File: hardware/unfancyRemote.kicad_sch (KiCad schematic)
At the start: 50 parts, among them J3 HALL1/PPM, J4 HALL2, J6 VIN, J7 VBAT, J8 Motor, Q1 AO3401A, Q2 MMBT3904, Q3 MMBT3904, SW1 SW_Push, U1 E28-2G4M12S, U2 MCP73871-2AA, U3 ESP32-C3_SUPERMINI

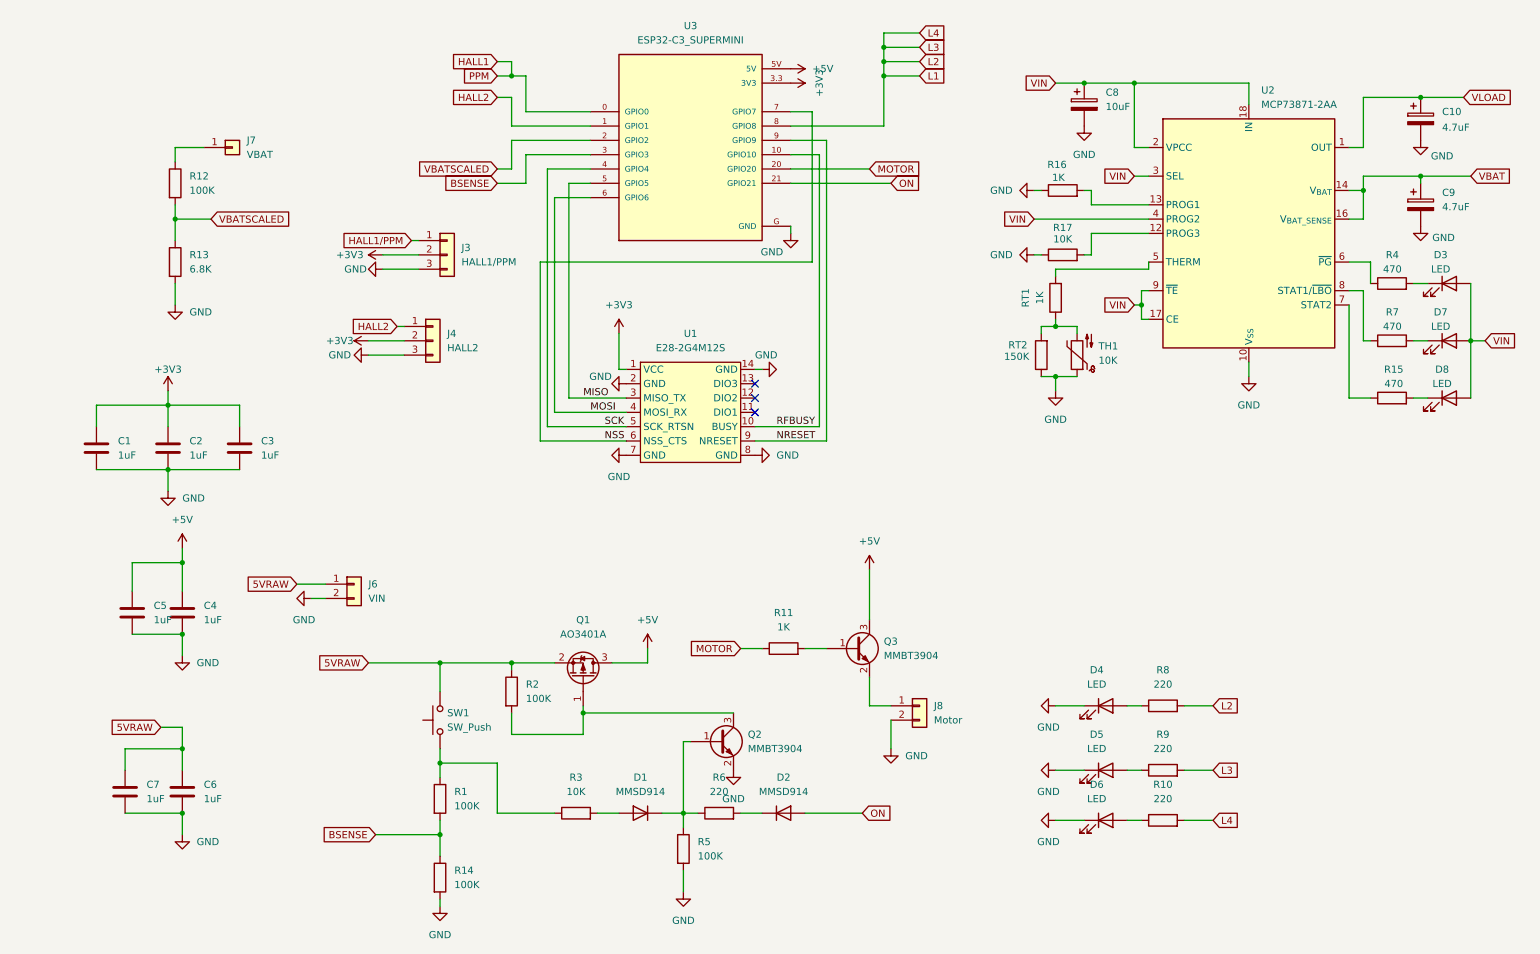
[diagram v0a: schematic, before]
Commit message: power progress
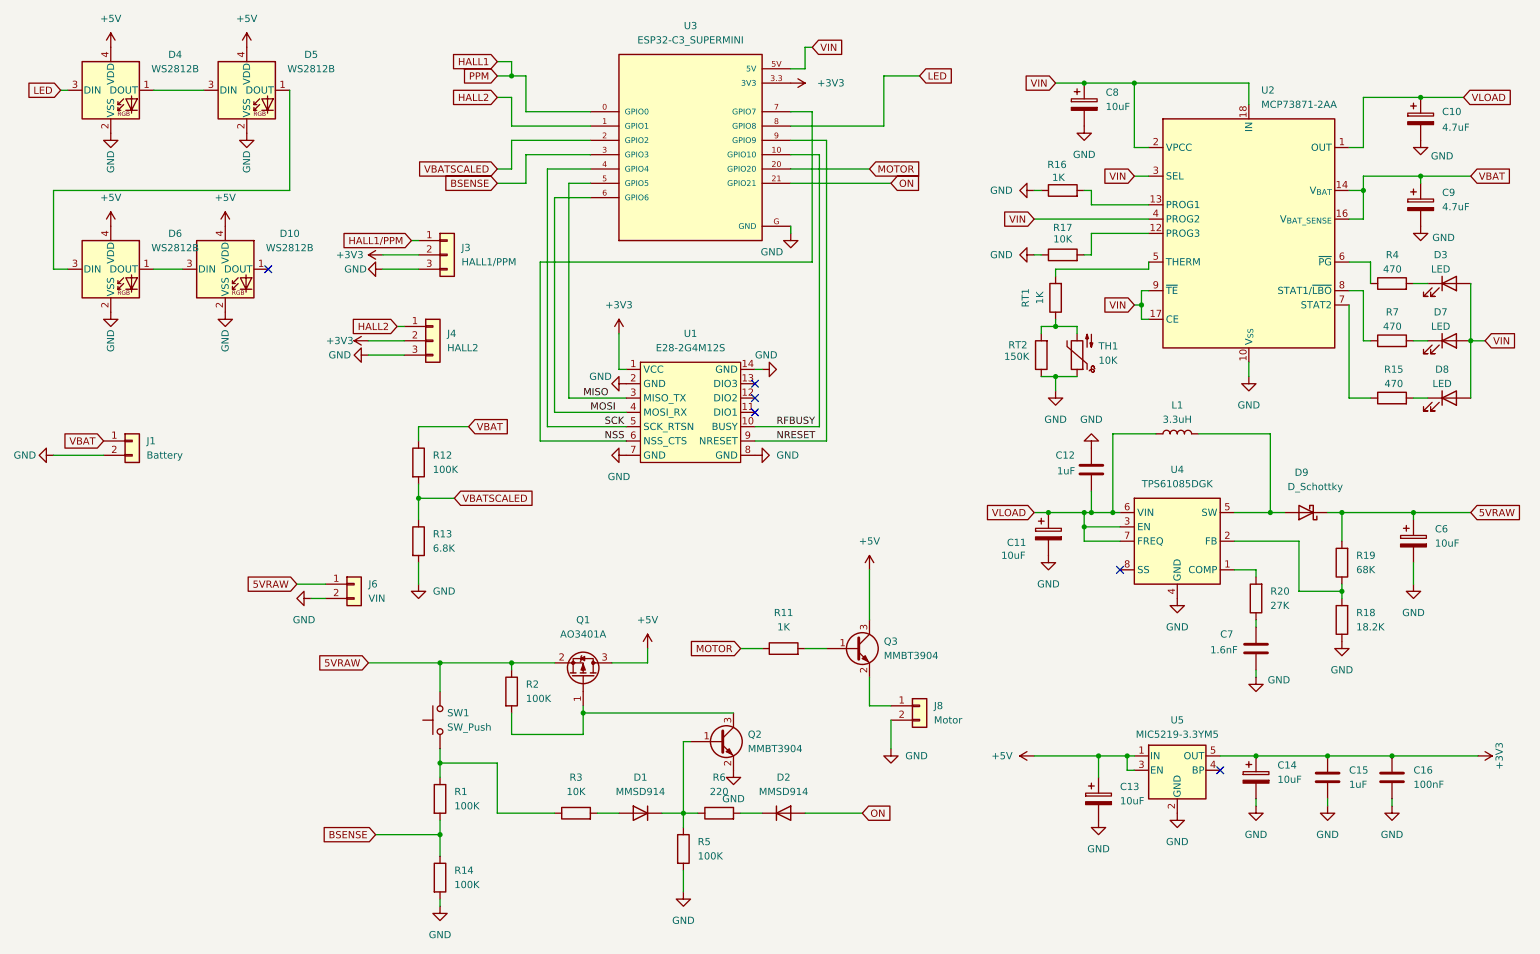
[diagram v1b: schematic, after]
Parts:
- removed C1, C2, C3, C4, C5, C6: 1uF, Capacitor_SMD:C_0603_1608Metric, symbol Device:C
- removed D4, D5, D6: LED, LED_SMD:LED_0805_2012Metric, symbol Device:LED
- removed J7: VBAT, Connector_wire:SolderWirePad_1x01_SMD_1x2mm, symbol Connector_Generic:Conn_01x01
- removed R10, R8, R9: 220, Resistor_SMD:R_0603_1608Metric, symbol Device:R
- added C11, C13, C14, C6: 10uF, Capacitor_Tantalum_SMD:CP_EIA-3216-10_Kemet-I, symbol Device:C_Polarized
- added C12, C15: 1uF, Capacitor_SMD:C_0402_1005Metric, symbol Device:C
- added C16: 100nF, Capacitor_SMD:C_0402_1005Metric, symbol Device:C
- added D10, D4, D5, D6: WS2812B, LED_SMD:LED_WS2812B-2020_PLCC4_2.0x2.0mm, symbol LED:WS2812B-2020
- added D9: D_Schottky, Diode_SMD:D_SOD-523, symbol Device:D_Schottky
- added J1: Battery, unfancyRemote_components:SolderWirePad_1x02_SMD_1x2mm, symbol Connector_Generic:Conn_01x02
- added L1: 3.3uH, Inductor_SMD:L_01005_0402Metric, symbol Device:L
- added R18: 18.2K, Resistor_SMD:R_0402_1005Metric, symbol Device:R
- added R19: 68K, Resistor_SMD:R_0402_1005Metric, symbol Device:R
- added R20: 27K, Resistor_SMD:R_0402_1005Metric, symbol Device:R
- added U4: TPS61085DGK, Package_SO:VSSOP-8_3x3mm_P0.65mm, symbol Regulator_Switching:TPS61085DGK
- added U5: MIC5219-3.3YM5, Package_TO_SOT_SMD:SOT-23-5, symbol Regulator_Linear:MIC5219-3.3YM5
- C10, C8, C9: footprint (none) -> Capacitor_Tantalum_SMD:CP_EIA-3216-10_Kemet-I
- C7: value 1uF -> 1.6nF; footprint Capacitor_SMD:C_0603_1608Metric -> Capacitor_SMD:C_0402_1005Metric
- R1, R11, R12, R13, R14, R15, R16, R17, R2, R3, R4, R5, R6, R7, RT1, RT2: footprint Resistor_SMD:R_0603_1608Metric -> Resistor_SMD:R_0402_1005Metric
- TH1: footprint (none) -> Resistor_SMD:R_0402_1005Metric
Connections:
- net +3V3: now also C14.1, C15.1, C16.1, U5.5 (OUT)
- net +5V: now also C13.1, D10.4 (VDD), D4.4 (VDD), D5.4 (VDD), D6.4 (VDD), U5.1 (IN), U5.3 (EN); no longer U3.5V
- net 5VRAW: now also C6.1, D9.1 (K), R19.2; no longer C7.1
- net GND: now also C11.2, C12.1, C13.2, C14.2, C15.2, C16.2, C6.2, D10.2 (VSS), D4.2 (VSS), D5.2 (VSS), D6.2 (VSS), J1.2 (Pin_2), R18.1, U4.4 (GND), U5.2 (GND)
- net VBAT: now also R12.1, J1.1 (Pin_1)
- net VIN: now also U3.5V
- net VLOAD: now also C11.1, C12.2, L1.1, U4.3 (EN), U4.6 (VIN), U4.7 (FREQ)
- net L1 renamed LED
- net LED: now also D4.3 (DIN)
- new net: R18.2, R19.1, U4.2 (FB)
- new net: C7.1, R20.1
- new net: D9.2 (A), L1.2, U4.5 (SW)
- new net: D10.3 (DIN), D6.1 (DOUT)
- new net: D4.1 (DOUT), D5.3 (DIN)
- new net: D5.1 (DOUT), D6.3 (DIN)
- new net: R20.2, U4.1 (COMP)
- no-connect marks 3 -> 6
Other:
- moved on the sheet: R12, R13

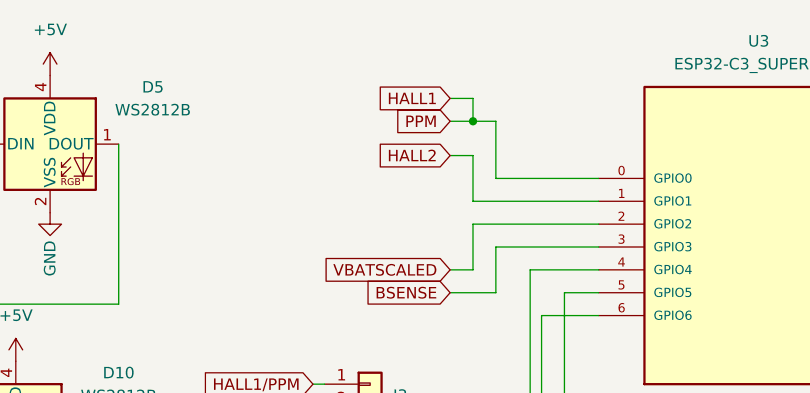
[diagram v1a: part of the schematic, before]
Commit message: routing
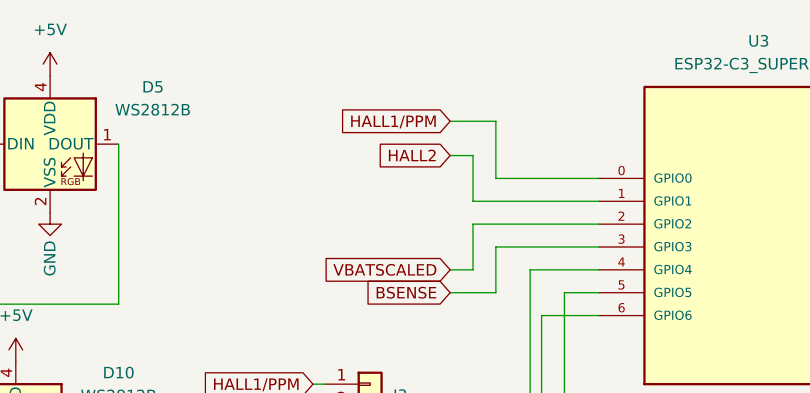
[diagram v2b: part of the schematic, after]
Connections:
- net HALL1 is gone; now on net HALL1/PPM: U3.0 (GPIO0)
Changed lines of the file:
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@@
-	)
-	(junction
-		(at 104.14 25.4)
-		(diameter 0)
-		(color 0 0 0 0)
 	)
 	(junction
@@
 	(wire
 		(pts
-			(xy 101.6 22.86) (xy 104.14 22.86)
-		)
-		(stroke
-			(width 0)
-			(type default)
-		)
-	)
-	(wire
-		(pts
 			(xy 110.49 41.91) (xy 118.11 41.91)
 		)
@@
 	(wire
 		(pts
-			(xy 106.68 25.4) (xy 104.14 25.4)
-		)
-		(stroke
-			(width 0)
-			(type default)
-		)
-	)
-	(wire
-		(pts
 			(xy 81.28 59.69) (xy 87.63 59.69)
 		)
@@
 	(wire
 		(pts
-			(xy 104.14 22.86) (xy 104.14 25.4)
-		)
-		(stroke
-			(width 0)
-			(type default)
-		)
-	)
-	(wire
-		(pts
 			(xy 176.53 25.4) (xy 170.18 25.4)
 		)
@@
 	(wire
 		(pts
-			(xy 101.6 25.4) (xy 104.14 25.4)
+			(xy 101.6 25.4) (xy 106.68 25.4)
 		)
 		(stroke
@@
 		)
 	)
-	(global_label "PPM"
+	(global_label "HALL1{slash}PPM"
 		(shape input)
 		(at 101.6 25.4 180)
@@
 		)
 		(property "Intersheetrefs" "${INTERSHEET_REFS}"
-			(at 94.6234 25.4 0)
+			(at 87.6081 25.4 0)
 			(effects
 				(font
@@
 			(effects
 				(font
-					(size 1.27 1.27)
-				)
-				(justify right)
-				(hide yes)
-			)
-		)
-	)
-	(global_label "HALL1"
-		(shape input)
-		(at 101.6 22.86 180)
-		(fields_autoplaced yes)
-		(effects
-			(font
-				(size 1.27 1.27)
-			)
-			(justify right)
-		)
-		(property "Intersheetrefs" "${INTERSHEET_REFS}"
-			(at 92.93 22.86 0)
-			(effects
-				(font
